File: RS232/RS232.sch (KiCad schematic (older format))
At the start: 31 parts

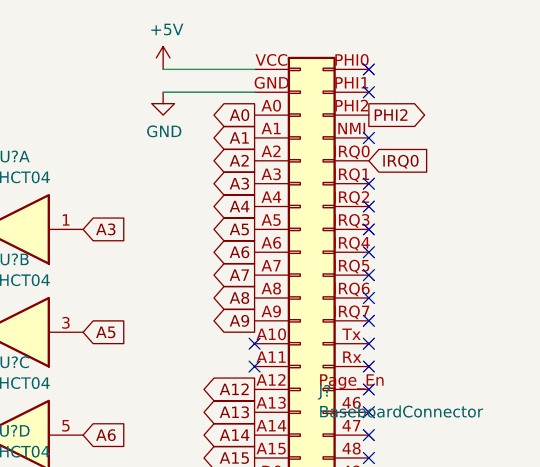
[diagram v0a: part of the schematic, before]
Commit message: Fixed bugs...
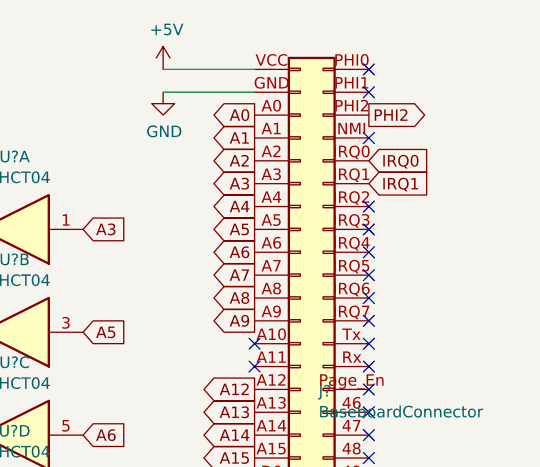
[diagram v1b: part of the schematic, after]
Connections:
- net IRQ1: now also J?.IRQ1
- no-connect marks 48 -> 47
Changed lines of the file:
@@
 NoConn ~ 10600 1500
 NoConn ~ 10600 1400
-NoConn ~ 10600 1300
 NoConn ~ 10600 1100
 NoConn ~ 10600 900
@@
 Wire Wire Line
 	4300 4200 4550 4200
+Text GLabel 10600 1300 2    50   Input ~ 0
+IRQ1
 $EndSCHEMATC
